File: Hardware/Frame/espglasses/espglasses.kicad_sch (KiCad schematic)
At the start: 0 parts

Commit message: kicad start
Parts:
- added C1: 10uF, symbol Device:C
- added C2: 100nF, symbol Device:C
- added D1: GREEN, symbol Device:LED
- added J1: BATTERY_1S, symbol Connector_Generic:Conn_01x02
- added J2: OLED_SH1106_I2C, symbol Connector_Generic:Conn_01x04
- added J3: TOUCH_INPUTS, symbol Connector_Generic:Conn_01x02
- added J4: AUDIO_OUT_MONO, symbol Connector_Generic:Conn_01x02
- added J5: UART_BOOT_DEBUG, symbol Connector_Generic:Conn_01x06
- added J6: LED_STATUS, symbol Connector_Generic:Conn_01x02
- added R1: 1k, symbol Device:R
- added R2, R3: 10k, symbol Device:R
- added U1: ESP32_DEV_BOARD_PIN_BREAKOUT, symbol Connector_Generic:Conn_02x19_Odd_Even
- added _TEMPLATE_C: C_TEMPLATE, symbol Device:C
- added _TEMPLATE_D: LED_TEMPLATE, symbol Device:LED
- added _TEMPLATE_R: R_TEMPLATE, symbol Device:R
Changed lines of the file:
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@@
-(kicad_sch
-	(version 20250114)
-	(generator "eeschema")
-	(generator_version "9.0")
-	(paper "A4")
-	(sheet_instances
-		(path "/"
-			(page "1")
-		)
-	)
-	(embedded_fonts no)
-)

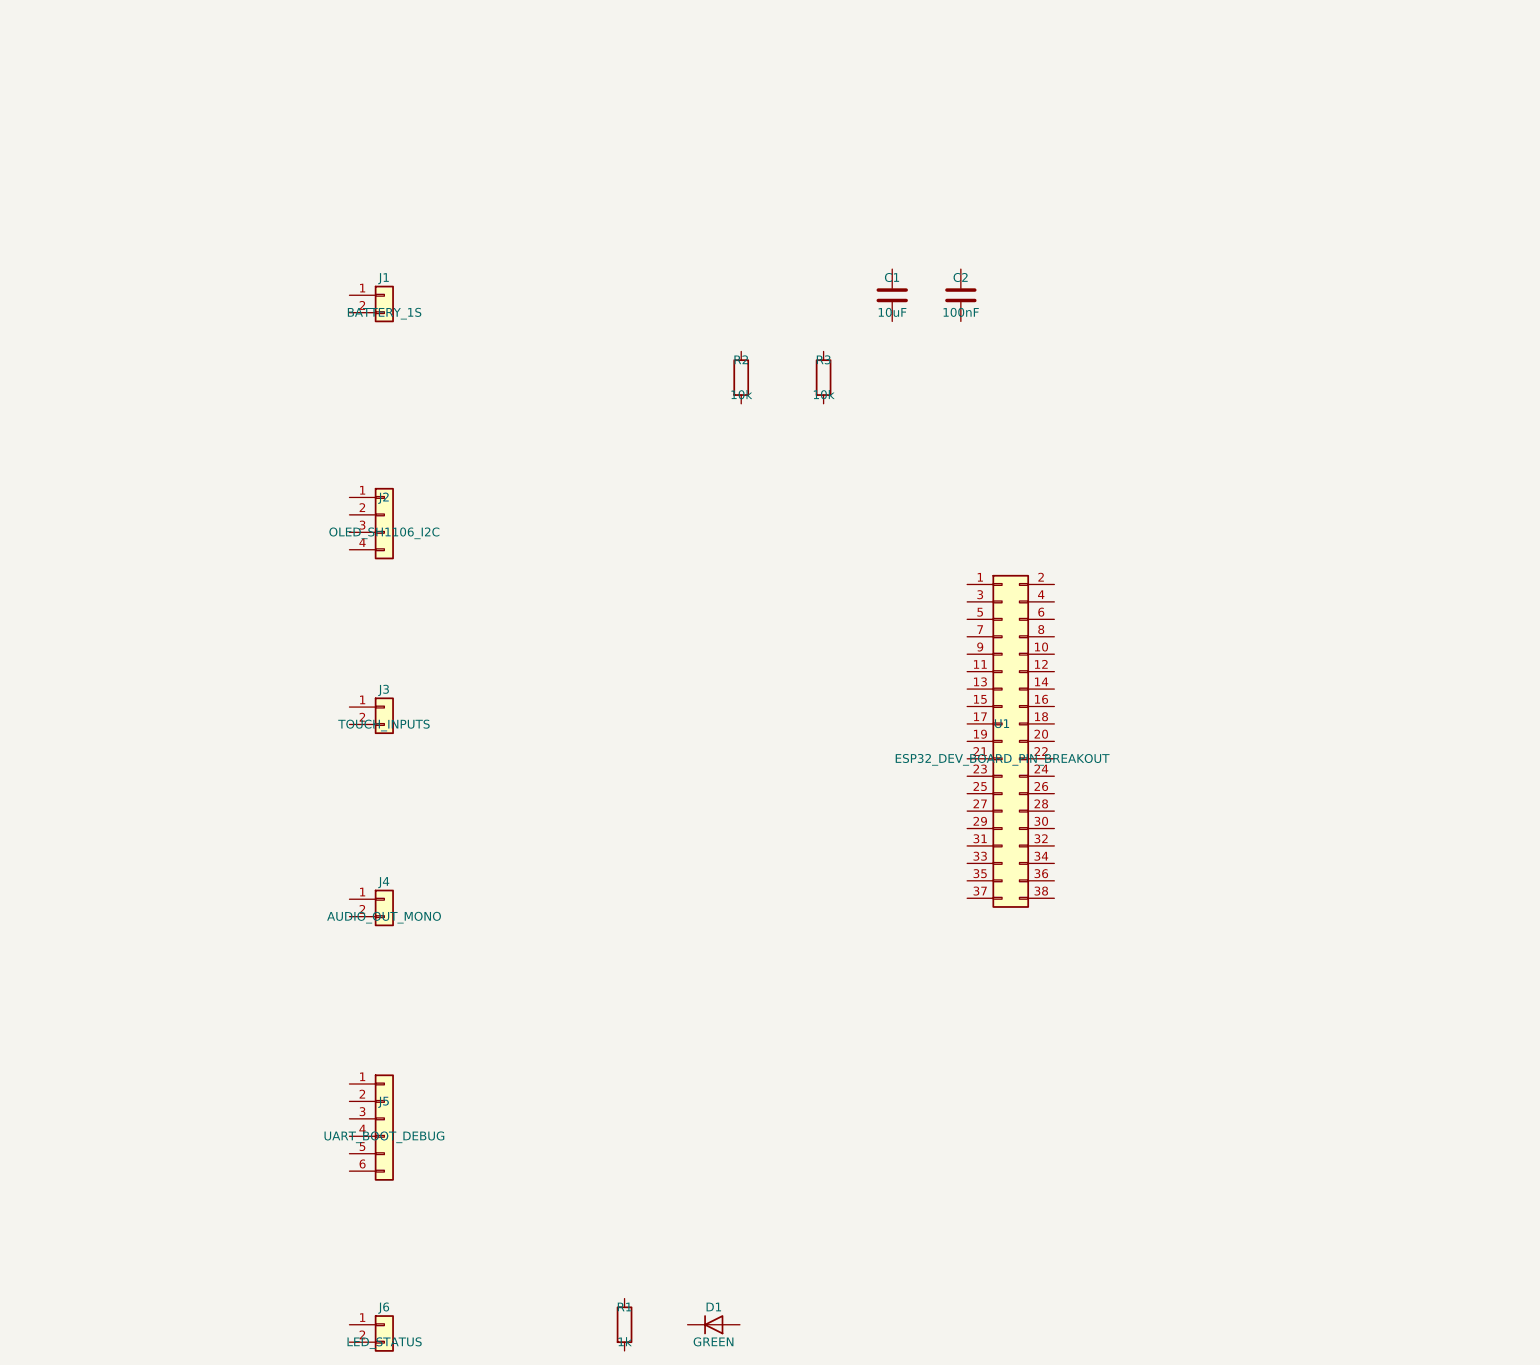
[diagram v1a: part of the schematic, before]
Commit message: kicad checkpoint
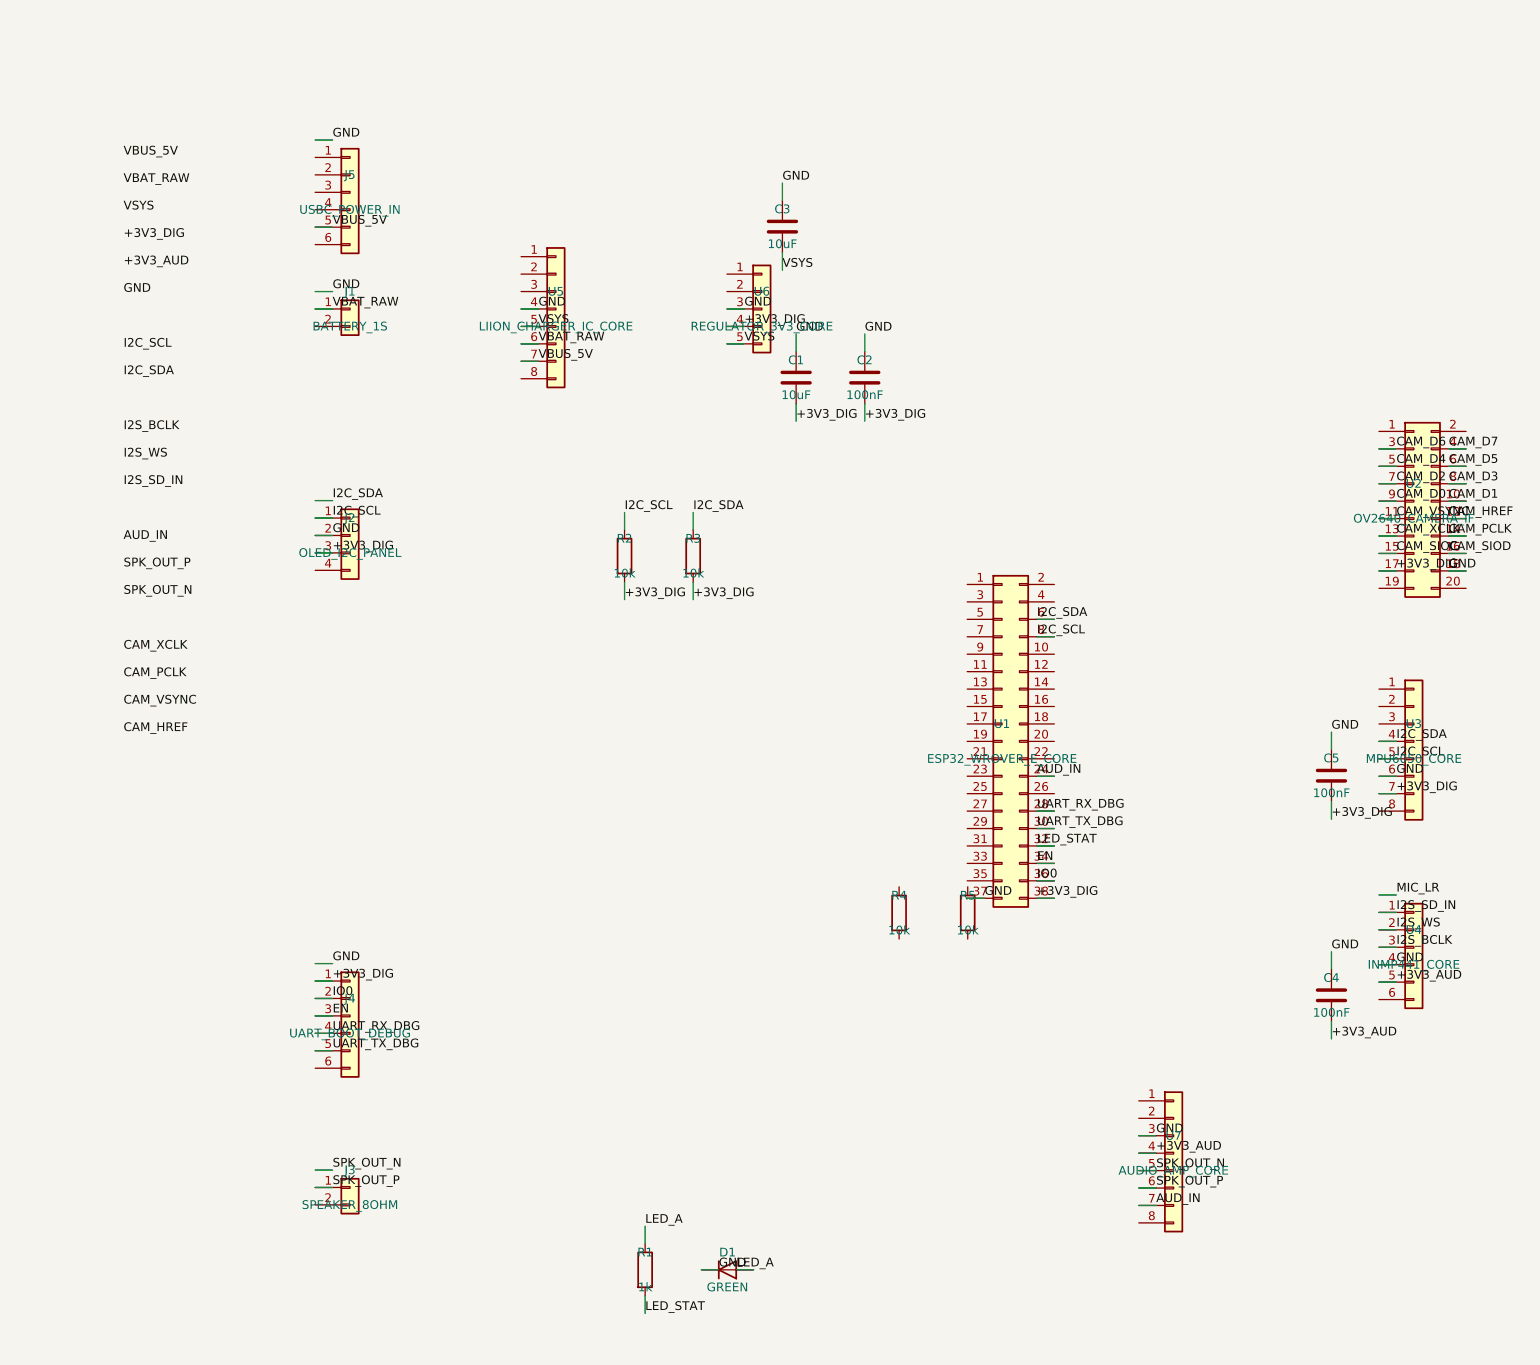
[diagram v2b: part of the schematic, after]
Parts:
- removed J4: AUDIO_OUT_MONO, symbol Connector_Generic:Conn_01x02
- removed J6: LED_STATUS, symbol Connector_Generic:Conn_01x02
- added C3: 10uF, Capacitor_SMD:C_0603_1608Metric, symbol Device:C
- added C4, C5: 100nF, Capacitor_SMD:C_0603_1608Metric, symbol Device:C
- added J4: UART_BOOT_DEBUG, Connector_PinHeader_2.54mm:PinHeader_1x06_P2.54mm_Vertical, symbol Connector_Generic:Conn_01x06
- added R4, R5: 10k, Resistor_SMD:R_0603_1608Metric, symbol Device:R
- added U2: OV2640_CAMERA_IF, Connector_FFC-FPC:TE_1734839-0_1x20-1MP_P0.5mm_Horizontal, symbol Connector_Generic:Conn_02x10_Odd_Even
- added U3: MPU6050_CORE, Package_QFN:QFN-24-1EP_4x4mm_P0.5mm_EP2.6x2.6mm, symbol Connector_Generic:Conn_01x08
- added U4: INMP441_CORE, Package_LGA:LGA-6_3x4mm_P0.5mm, symbol Connector_Generic:Conn_01x06
- added U5: LIION_CHARGER_IC_CORE, Package_SO:SOIC-8_3.9x4.9mm_P1.27mm, symbol Connector_Generic:Conn_01x08
- added U6: REGULATOR_3V3_CORE, Package_TO_SOT_SMD:SOT-223-3_TabPin2, symbol Connector_Generic:Conn_01x05
- added U7: AUDIO_AMP_CORE, Package_SO:SOIC-16_3.9x9.9mm_P1.27mm, symbol Connector_Generic:Conn_01x08
- C1, C2: footprint (none) -> Capacitor_SMD:C_0603_1608Metric
- D1: footprint (none) -> LED_SMD:LED_0603_1608Metric
- J1: footprint (none) -> Connector_JST:JST_PH_B2B-PH-K_1x02_P2.00mm_Vertical
- J2: value OLED_SH1106_I2C -> OLED_I2C_PANEL; footprint (none) -> Connector_PinHeader_2.54mm:PinHeader_1x04_P2.54mm_Vertical
- J3: value TOUCH_INPUTS -> SPEAKER_8OHM; footprint (none) -> Connector_PinHeader_2.54mm:PinHeader_1x02_P2.54mm_Vertical
- J5: value UART_BOOT_DEBUG -> USBC_POWER_IN; footprint (none) -> Connector_USB:USB_C_Receptacle_HRO_TYPE-C-31-M-12
- R1, R2, R3: footprint (none) -> Resistor_SMD:R_0603_1608Metric
- U1: value ESP32_DEV_BOARD_PIN_BREAKOUT -> ESP32_WROVER_E_CORE; footprint (none) -> RF_Module:ESP32-WROVER-E
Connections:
- net VBUS_5V: now reaches J5.5 (Pin_5)
- net VBUS_5V: now also U5.7 (Pin_7)
- net I2C_SCL: now reaches J2.1 (Pin_1)
- net I2C_SCL: now also R2.1, U1.8 (Pin_8), U3.5 (Pin_5)
- net GND: now reaches J2.2 (Pin_2)
- net GND: now also C1.1, C2.1, D1.1 (K), U1.37 (Pin_37), C3.1, C4.1, C5.1, U2.18 (Pin_18), U3.6 (Pin_6), U4.4 (Pin_4), U5.4 (Pin_4), U6.3 (Pin_3), U7.3 (Pin_3)
- net +3V3_DIG: now reaches J2.3 (Pin_3)
- net +3V3_DIG: now also C1.2, C2.2, R2.2, R3.2, U1.38 (Pin_38), C5.2, J4.1 (Pin_1), U2.17 (Pin_17), U3.7 (Pin_7), U6.4 (Pin_4)
- net I2C_SDA: now reaches R3.1
- net I2C_SDA: now also U1.6 (Pin_6), U3.4 (Pin_4)
- net AUD_IN: now reaches U1.24 (Pin_24)
- net AUD_IN: now also U7.7 (Pin_7)
- net UART_RX_DBG: now reaches U1.28 (Pin_28)
- net UART_RX_DBG: now also J4.4 (Pin_4)
- net UART_TX_DBG: now reaches U1.30 (Pin_30)
- net UART_TX_DBG: now also J4.5 (Pin_5)
- net LED_STAT: now reaches U1.32 (Pin_32)
- net LED_STAT: now also R1.2
- net EN: now reaches U1.34 (Pin_34)
- net EN: now also J4.3 (Pin_3)
- net IO0: now reaches U1.36 (Pin_36)
- net IO0: now also J4.2 (Pin_2)
- net VBAT_RAW: now reaches J1.1 (Pin_1)
- net VBAT_RAW: now also U5.6 (Pin_6)
- net SPK_OUT_P: now reaches J3.1 (Pin_1)
- net SPK_OUT_P: now also U7.6 (Pin_6)
- net LED_A: now reaches D1.2 (A)
- net LED_A: now also R1.1
- new net +3V3_AUD: C4.2, U4.5 (Pin_5), U7.4 (Pin_4)
- new net CAM_D0: U2.9 (Pin_9)
- new net CAM_D1: U2.10 (Pin_10)
- new net CAM_D2: U2.7 (Pin_7)
- new net CAM_D3: U2.8 (Pin_8)
- new net CAM_D4: U2.5 (Pin_5)
- new net CAM_D5: U2.6 (Pin_6)
- new net CAM_D6: U2.3 (Pin_3)
- new net CAM_D7: U2.4 (Pin_4)
- new net CAM_HREF: U2.12 (Pin_12)
- new net CAM_PCLK: U2.14 (Pin_14)
- new net CAM_SIOC: U2.15 (Pin_15)
- new net CAM_SIOD: U2.16 (Pin_16)
- new net CAM_VSYNC: U2.11 (Pin_11)
- new net CAM_XCLK: U2.13 (Pin_13)
- new net I2S_BCLK: U4.3 (Pin_3)
- new net I2S_SD_IN: U4.1 (Pin_1)
- new net I2S_WS: U4.2 (Pin_2)
- new net SPK_OUT_N: U7.5 (Pin_5)
- new net VSYS: C3.2, U5.5 (Pin_5), U6.5 (Pin_5)
